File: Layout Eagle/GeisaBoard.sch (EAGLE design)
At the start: 19 parts, among them X1 22-23-2021

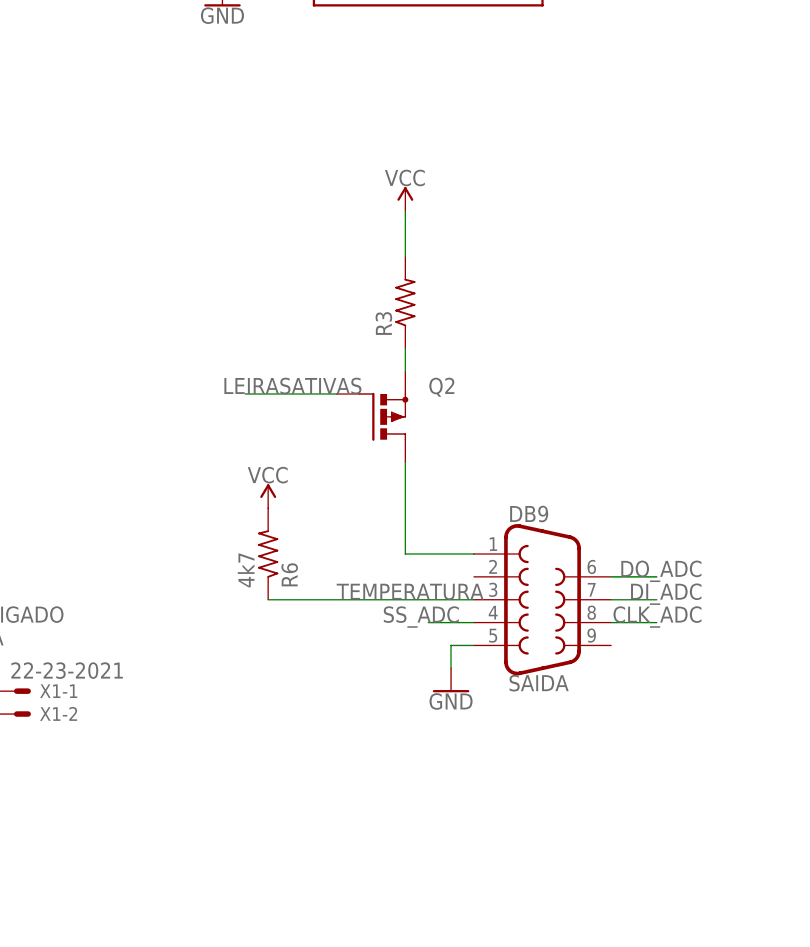
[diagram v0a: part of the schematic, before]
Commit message: GeisaBoard layout completo (espero)
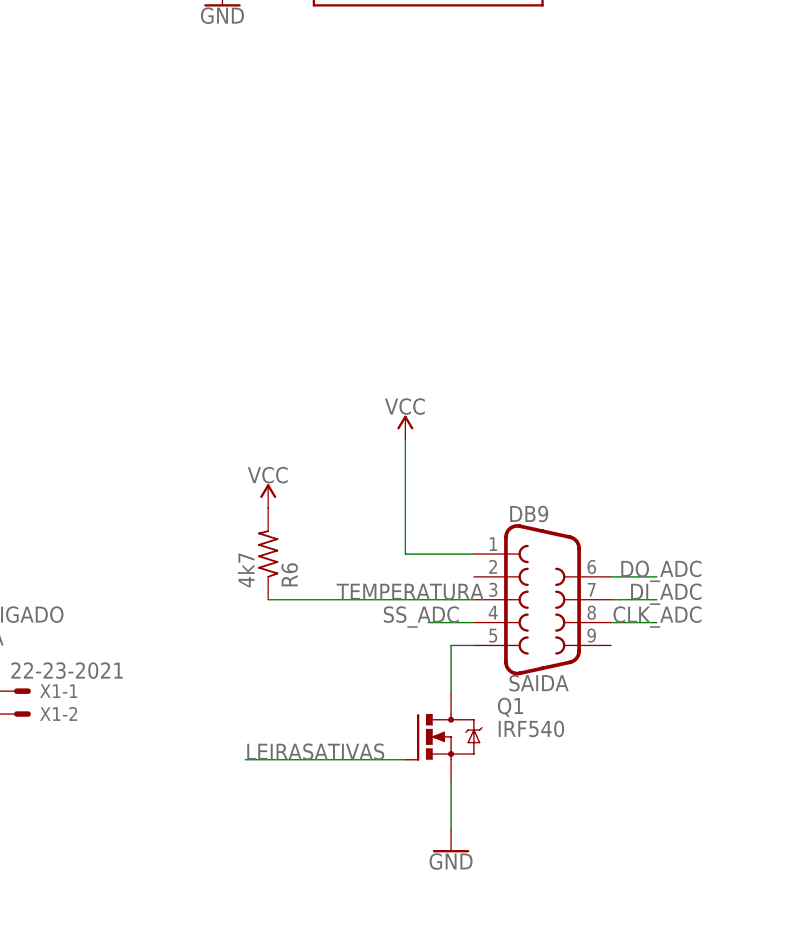
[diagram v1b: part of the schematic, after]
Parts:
- removed Q2: (no value), transistor-power:PMOSFET_PTO220BV
- removed R3: (no value), rcl:R-US_0204/7
- added Q1: IRF540, transistor-power:IRF540
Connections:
- removed net N$1: DB9.1, Q2.D
- net GND: now also Q1.S; no longer DB9.5
- net LEIRASATIVAS: now also Q1.G; no longer Q2.G
- net N$2: now also DB9.5, Q1.D; no longer Q2.S, R3.1
- net VCC: now also DB9.1; no longer R3.2
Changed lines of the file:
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@@
 <part name="X1" library="con-molex" library_urn="urn:adsk.eagle:library:165" deviceset="22-23-2021" device=""/>
 <part name="FRAME1" library="frames" library_urn="urn:adsk.eagle:library:229" deviceset="DINA4_L" device=""/>
-<part name="R3" library="rcl" library_urn="urn:adsk.eagle:library:334" deviceset="R-US_" device="0204/7" package3d_urn="urn:adsk.eagle:package:23498/1"/>
-<part name="Q2" library="transistor-power" library_urn="urn:adsk.eagle:library:400" deviceset="PMOSFET_P" device="TO220BV" package3d_urn="urn:adsk.eagle:package:29484/3"/>
+<part name="Q1" library="transistor-power" library_urn="urn:adsk.eagle:library:400" deviceset="IRF540" device="" package3d_urn="urn:adsk.eagle:package:29484/3"/>
 </parts>
 <sheets>
@@
 <instance part="R9" gate="G$1" x="-109.22" y="53.34" rot="R90"/>
 <instance part="RESET" gate="G$1" x="-109.22" y="40.64"/>
-<instance part="GND6" gate="1" x="25.4" y="10.16" rot="MR0"/>
-<instance part="SUPPLY9" gate="G$1" x="20.32" y="63.5"/>
+<instance part="GND6" gate="1" x="25.4" y="-7.62" rot="MR0"/>
+<instance part="SUPPLY9" gate="G$1" x="20.32" y="38.1"/>
 <instance part="GND12" gate="1" x="76.2" y="91.44"/>
 <instance part="GND13" gate="1" x="-96.52" y="-12.7"/>
@@
 <instance part="FRAME1" gate="G$1" x="-137.16" y="-50.8"/>
 <instance part="FRAME1" gate="G$2" x="25.4" y="-50.8"/>
-<instance part="R3" gate="G$1" x="20.32" y="53.34" rot="R90"/>
-<instance part="Q2" gate="G$1" x="17.78" y="40.64"/>
+<instance part="Q1" gate="G$1" x="22.86" y="5.08"/>
 </instances>
 <busses>
@@
 </segment>
 <segment>
-<wire x1="12.7" y1="43.18" x2="2.54" y2="43.18" width="0.1524" layer="91"/>
-<label x="0" y="43.18" size="1.778" layer="95"/>
-<pinref part="Q2" gate="G$1" pin="G"/>
+<pinref part="Q1" gate="G$1" pin="G"/>
+<wire x1="20.32" y1="2.54" x2="2.54" y2="2.54" width="0.1524" layer="91"/>
+<label x="2.54" y="2.54" size="1.778" layer="95"/>
 </segment>
 </net>
@@
 </segment>
 <segment>
-<pinref part="GND6" gate="1" pin="GND"/>
-<wire x1="25.4" y1="15.24" x2="25.4" y2="12.7" width="0.1524" layer="91"/>
-<pinref part="DB9" gate="G$1" pin="5"/>
-<wire x1="27.94" y1="15.24" x2="25.4" y2="15.24" width="0.1524" layer="91"/>
-</segment>
-<segment>
 <pinref part="GND17" gate="1" pin="GND"/>
 <wire x1="86.36" y1="30.48" x2="93.98" y2="30.48" width="0.1524" layer="91"/>
@@
 <wire x1="-83.82" y1="86.36" x2="-91.44" y2="86.36" width="0.1524" layer="91"/>
 <wire x1="-91.44" y1="86.36" x2="-91.44" y2="78.74" width="0.1524" layer="91"/>
+</segment>
+<segment>
+<pinref part="Q1" gate="G$1" pin="S"/>
+<pinref part="GND6" gate="1" pin="GND"/>
+<wire x1="25.4" y1="0" x2="25.4" y2="-5.08" width="0.1524" layer="91"/>
 </segment>
 </net>
@@
 </segment>
 <segment>
-<pinref part="R3" gate="G$1" pin="2"/>
+<wire x1="27.94" y1="25.4" x2="20.32" y2="25.4" width="0.1524" layer="91"/>
+<pinref part="DB9" gate="G$1" pin="1"/>
+<wire x1="20.32" y1="25.4" x2="20.32" y2="38.1" width="0.1524" layer="91"/>
 <pinref part="SUPPLY9" gate="G$1" pin="VCC"/>
-<wire x1="20.32" y1="58.42" x2="20.32" y2="63.5" width="0.1524" layer="91"/>
 </segment>
 </net>
@@
 </segment>
 </net>
-<net name="N$1" class="1">
-<segment>
-<wire x1="27.94" y1="25.4" x2="20.32" y2="25.4" width="0.1524" layer="91"/>
-<pinref part="DB9" gate="G$1" pin="1"/>
-<wire x1="20.32" y1="25.4" x2="20.32" y2="35.56" width="0.1524" layer="91"/>
-<pinref part="Q2" gate="G$1" pin="D"/>
-</segment>
-</net>
-<net name="N$2" class="0">
-<segment>
-<pinref part="R3" gate="G$1" pin="1"/>
-<wire x1="20.32" y1="45.72" x2="20.32" y2="48.26" width="0.1524" layer="91"/>
-<pinref part="Q2" gate="G$1" pin="S"/>
-</segment>
-</net>
+<net name="N$2" class="1">
+<segment>
+<pinref part="DB9" gate="G$1" pin="5"/>
+<wire x1="27.94" y1="15.24" x2="25.4" y2="15.24" width="0.1524" layer="91"/>
+<pinref part="Q1" gate="G$1" pin="D"/>
+<wire x1="25.4" y1="10.16" x2="25.4" y2="15.24" width="0.1524" layer="91"/>
+</segment>
+</net>
